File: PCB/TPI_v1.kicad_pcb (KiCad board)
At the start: 2 copper layers, 30 x 65 mm, 11 parts, among them J1 Raspberry pi zero w, J2 BME280, J3 BME280, U1 BMI160, U2 DS18B20

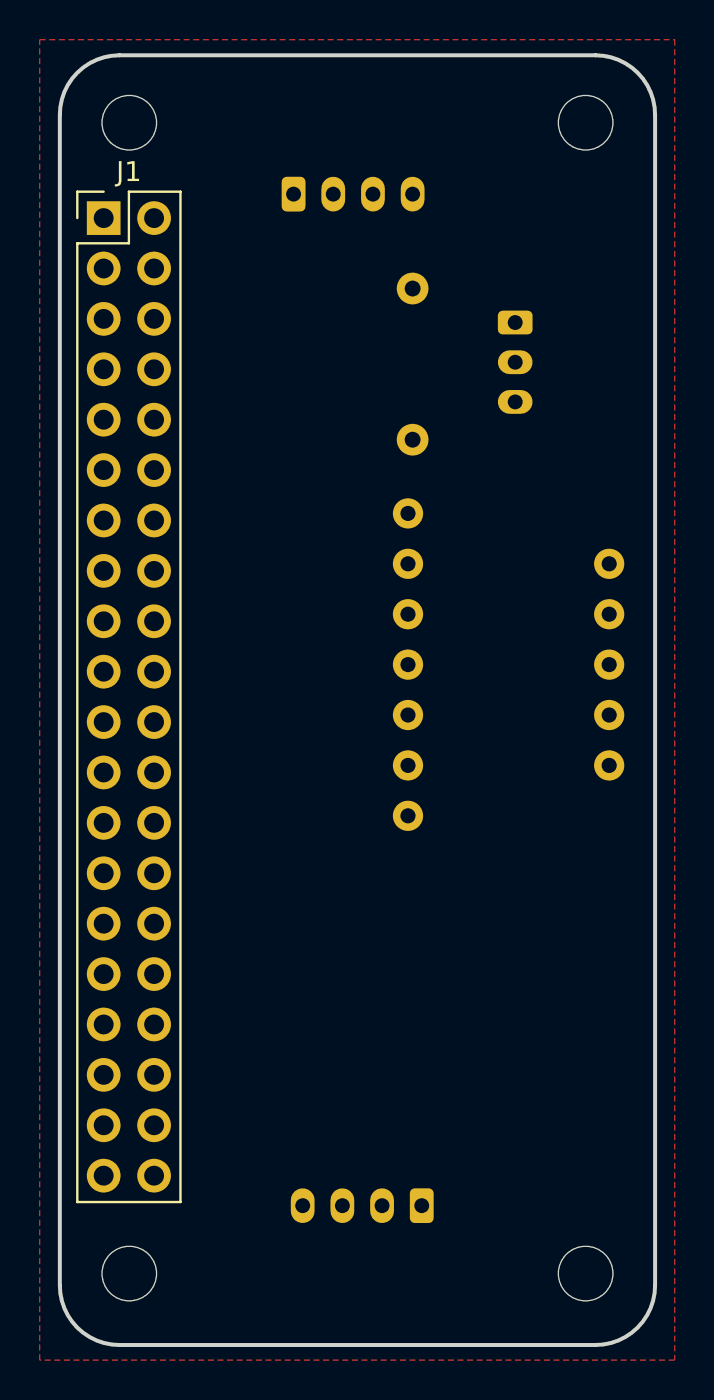
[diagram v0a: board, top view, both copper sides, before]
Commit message: PCB update
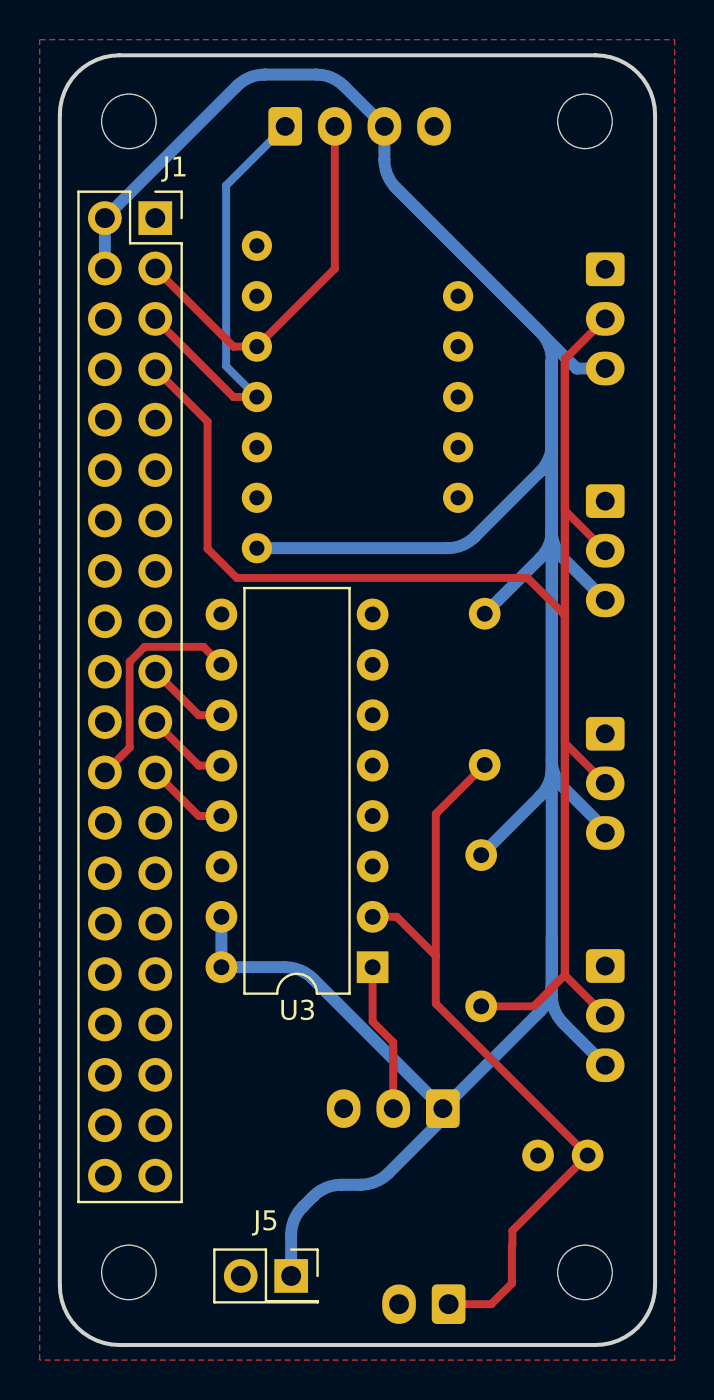
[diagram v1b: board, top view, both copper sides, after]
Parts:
- removed the ? at (171.0, 110.9)
- removed the ? at (148.0, 110.9)
- removed the ? at (171.0, 52.9)
- removed the ? at (148.0, 52.9)
- added ?: , , B.Cu at (171.0, 110.8)
- added ?: , , B.Cu at (148.0, 110.8)
- added ?: , , B.Cu at (171.0, 52.8)
- added ?: , , B.Cu at (148.0, 52.8)
- added C1: 100n, Capacitor_THT:C_Disc_D3.0mm_W1.6mm_P2.50mm, B.Cu at (171.1, 104.9)
- added G***: LOGO, Custom:Logo_TPI, F.Cu at (162.8, 108.0)
- added J4: MQ135, Connector_JST:JST_XH_B3B-XH-A_1x03_P2.50mm_Vertical, B.Cu at (163.8, 102.6)
- added J5: Buck, Connector_PinSocket_2.54mm:PinSocket_2x01_P2.54mm_Vertical, F.Cu at (156.2, 111.0)
- added R2: 10k, Resistor_THT:R_Axial_DIN0207_L6.3mm_D2.5mm_P7.62mm_Horizontal, B.Cu at (165.9, 77.6)
- added U3: MCP3008, Package_DIP:DIP-16_W7.62mm, F.Cu at (160.3, 95.5)
- added U4: DS18B20_2, Connector_JST:JST_XH_S3B-XH-A-1_1x03_P2.50mm_Horizontal, B.Cu at (172.0, 72.0)
- added U5: DS18B20_3, Connector_JST:JST_XH_S3B-XH-A-1_1x03_P2.50mm_Horizontal, B.Cu at (172.0, 60.3)
- added U6: DS18B20_4, Connector_JST:JST_XH_S3B-XH-A-1_1x03_P2.50mm_Horizontal, B.Cu at (172.0, 95.4)
- J2: footprint Connector_JST:JST_PH_S4B-PH-K_1x04_P2.00mm_Horizontal -> Connector_JST:JST_XH_S4B-XH-A-1_1x04_P2.50mm_Horizontal
- J3: value BME280 -> SIG2991; footprint Connector_JST:JST_PH_S4B-PH-K_1x04_P2.00mm_Horizontal -> Connector_JST:JST_XH_S2B-XH-A-1_1x02_P2.50mm_Horizontal
- U2: value DS18B20 -> DS18B20_1; footprint Connector_JST:JST_PH_S3B-PH-K_1x03_P2.00mm_Horizontal -> Connector_JST:JST_XH_S3B-XH-A-1_1x03_P2.50mm_Horizontal
- moved J3 56.5 mm to (164.1, 112.4), turned to 180 degrees
- moved J2 54.8 mm to (155.9, 53.1), turned to 0 degrees
- moved G*** 21.7 mm to (156.5, 86.9), turned to -90 degrees
- moved R1 21.2 mm to (165.7, 89.8), turned to -90 degrees
- moved U2 21.2 mm to (172.0, 83.7)
- moved U1 15.5 mm to (159.5, 66.7)
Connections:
- J1 pad 19: unconnected-(J1-GPIO10-Pad19) -> MOSI
- J1 pad 20: GND -> unconnected-(J1-GND-Pad20)
- J1 pad 21: unconnected-(J1-GPIO9-Pad21) -> MISO
- J1 pad 23: unconnected-(J1-GPIO11-Pad23) -> SCLK
- J1 pad 24: unconnected-(J1-GPIO8-Pad24) -> ~{CS}
- J1 pad 4: unconnected-(J1-5V-Pad4) -> +5V
- J3 pad 1: SCL -> ADC1
- J3 pad 2: SDA -> GND
- U1 pad 1: +3.3V -> +5V
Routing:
- net +5V: track 0.00 -> 207.6 mm
- net DQ: track 0.00 -> 122.0 mm
- net ADC1: track 0.00 -> 39.5 mm
- net SCL: track 0.00 -> 22.5 mm
- net SDA: track 0.00 -> 19.5 mm
- net ~{CS}: track 0.00 -> 11.4 mm
- net ADC0: track 0.00 -> 7.56 mm
- net SCLK: track 0.00 -> 4.24 mm
- net MOSI: track 0.00 -> 4.24 mm
- net MISO: track 0.00 -> 4.24 mm
